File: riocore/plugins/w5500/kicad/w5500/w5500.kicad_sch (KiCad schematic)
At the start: 34 parts, among them J6 RJ45_Pulse_J0011D21BNL, U8 W5500, Y2 Crystal_25MHz

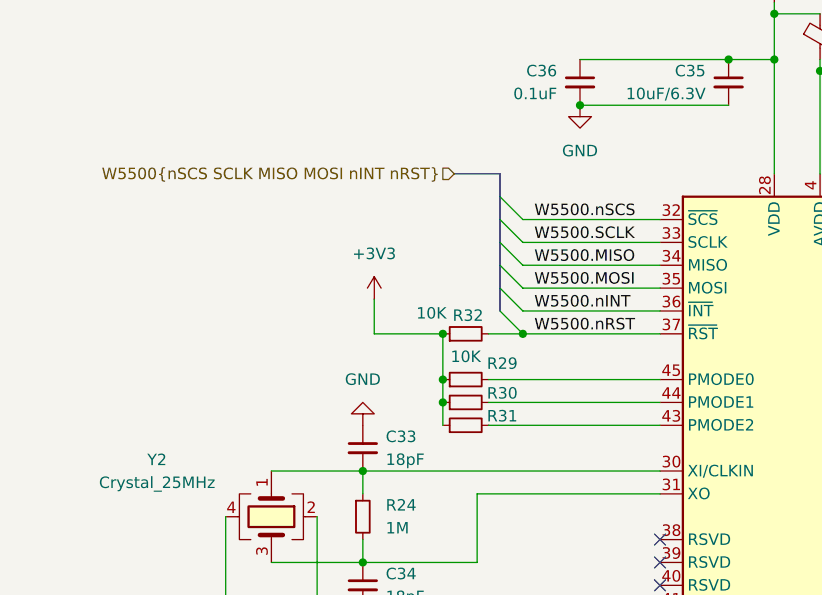
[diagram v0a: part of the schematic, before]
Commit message: kicad: fixes
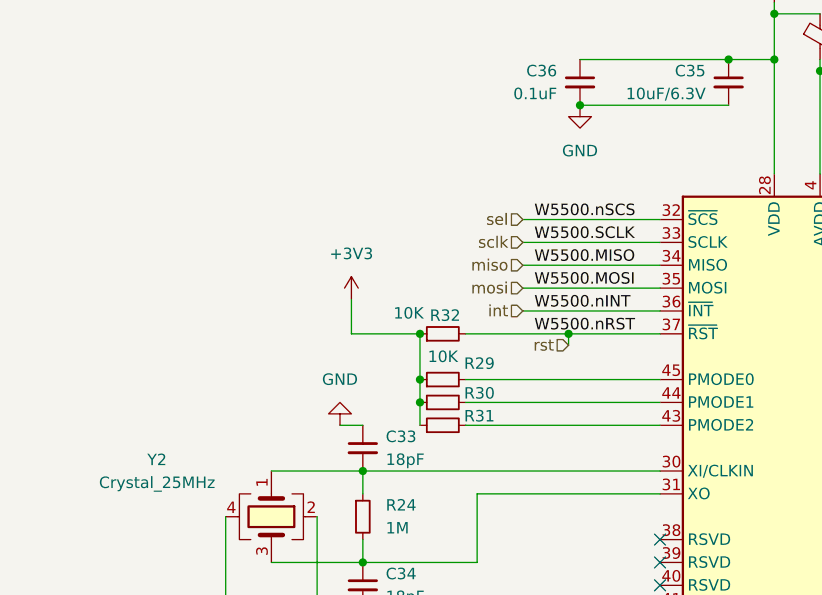
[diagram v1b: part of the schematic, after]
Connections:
- net W5500.MISO renamed miso
- net W5500.MOSI renamed mosi
- net W5500.SCLK renamed sclk
- net W5500.nINT renamed int
- net W5500.nRST renamed rst
- net W5500.nSCS renamed sel
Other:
- moved on the sheet: R29, R30, R31, R32
